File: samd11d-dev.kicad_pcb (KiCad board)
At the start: 2 copper layers, 30.5 x 29.2 mm, 24 parts, among them J1 Conn_02x05_Odd_Even, J2 USB_B_Micro, J3 Conn_01x08, J4 Conn_01x08, SW2 SW_Push, U1 ATSAMD11D14A-SS, U3 MCP1700-3302E_SOT23, U4 USBLC6-2SC6, Y1 32.768 kHz

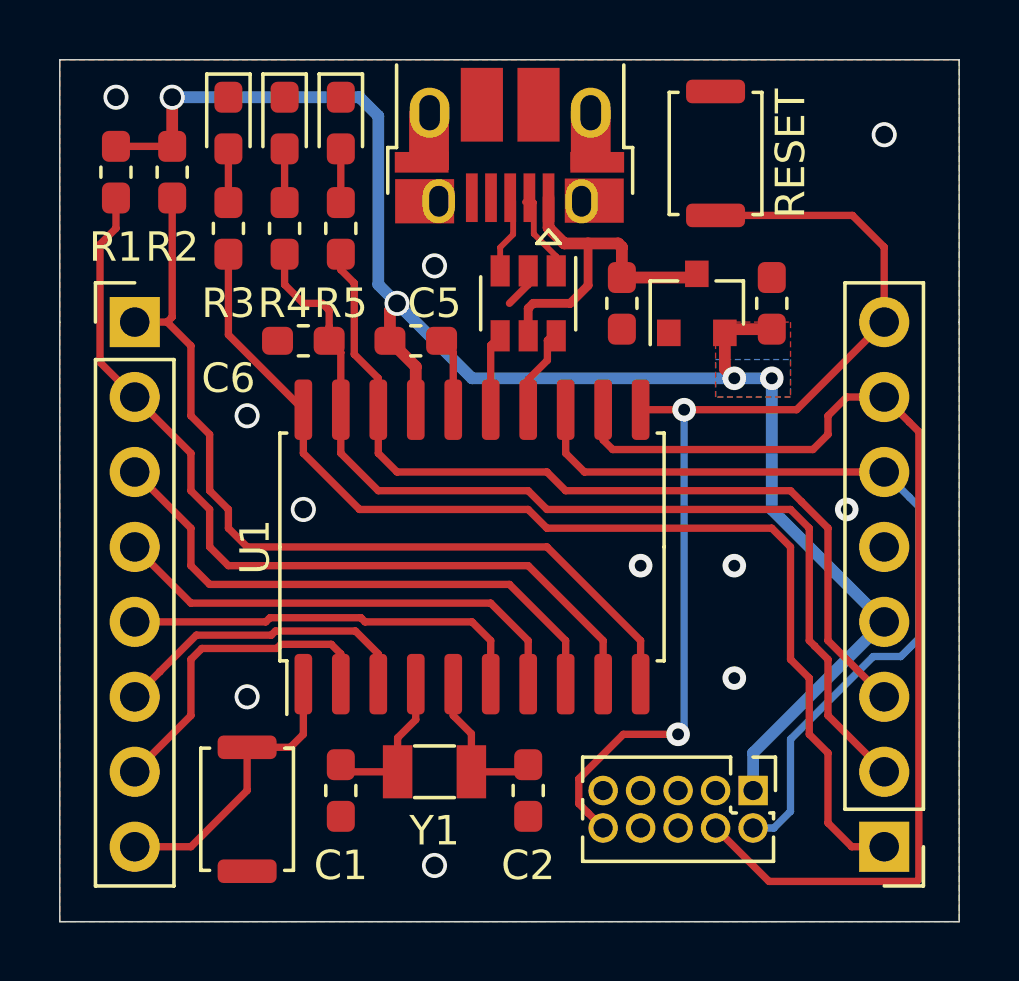
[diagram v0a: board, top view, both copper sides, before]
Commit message: First public release
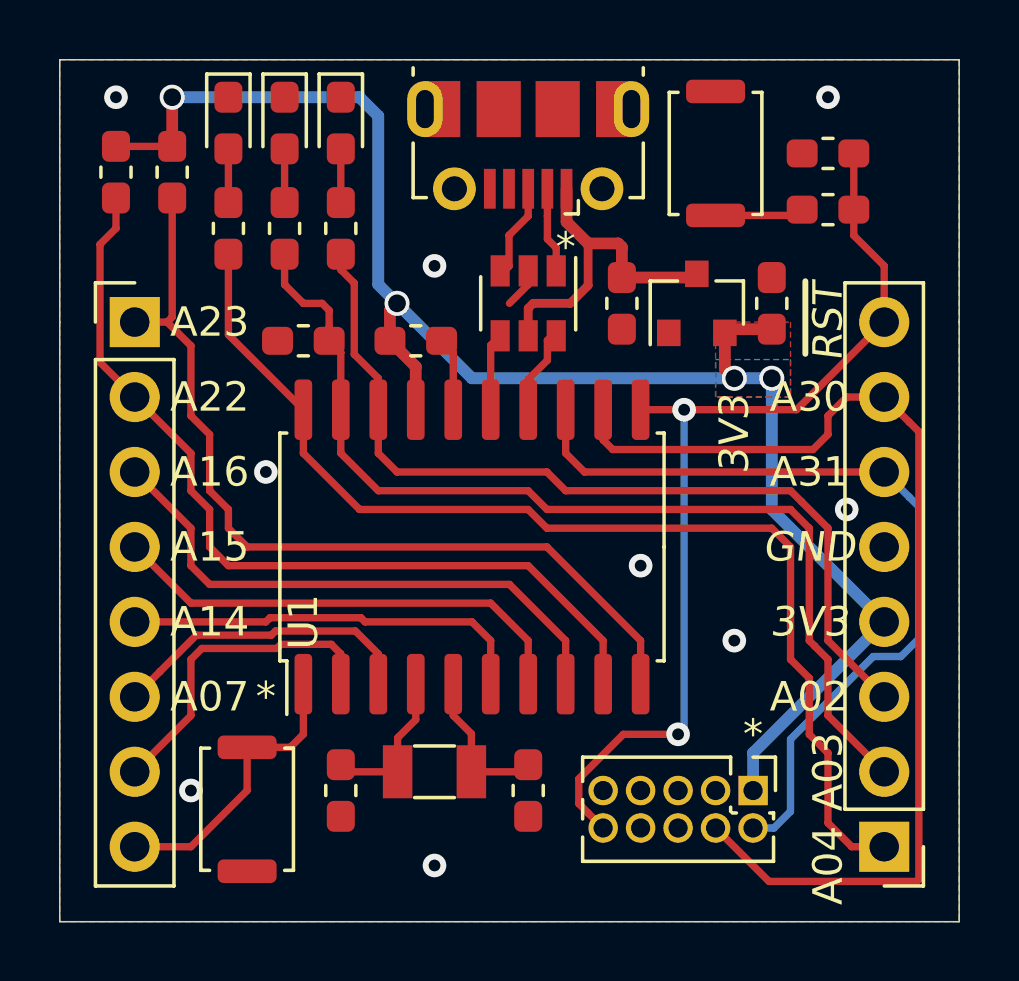
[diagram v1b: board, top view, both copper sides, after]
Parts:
- added C7: 100n, Capacitor_SMD:C_0603_1608Metric_Pad1.05x0.95mm_HandSolder, F.Cu at (153.0, 103.5)
- added R6: 330R, Resistor_SMD:R_0603_1608Metric_Pad1.05x0.95mm_HandSolder, F.Cu at (153.0, 105.4)
- added REF**: OSHW-Logo2_7.3x6mm_SilkScreen, Symbol:OSHW-Logo2_7.3x6mm_SilkScreen, B.Cu at (141.0, 116.2)
- J2: footprint Connector_USB:USB_Micro-B_Amphenol_10103594-0001LF_Horizontal -> Connector_USB:USB_Micro-B_Molex-105017-0001
- moved J2 0.63 mm to (142.9, 103.2)
- renumbered RESET to SW1
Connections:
- SW1 pad 1: /~RST -> Net-(R6-Pad1)
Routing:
- net Net-(R6-Pad1): track 0.00 -> 3.02 mm
- net /~RST: track 35.3 -> 32.7 mm
- net /USB_D+: track 2.70 -> 3.26 mm
- net GND: vias 11 -> 9
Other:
- board text added: "*"
- board text added: "3V3"
- board text added: "A02"
- board text added: "A03"
- board text added: "A04"
- board text added: "A05"
- board text added: "A06"
- board text added: "A07"
- board text added: "A14"
- board text added: "A15"
- board text added: "A16"
- board text added: "A22"
- board text added: "A23"
- board text added: "A30"
- board text added: "A31"
- board text added: "GND"
- board text added: "SAMD11D-dev v0.1"
- board text added: "awjlogan 2020"
- board text added: "~RST"
